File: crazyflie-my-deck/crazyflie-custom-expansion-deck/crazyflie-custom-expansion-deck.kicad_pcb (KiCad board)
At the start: 2 copper layers, 36.2 x 37.7 mm, 14 parts, among them J1 Conn_01x10, J2 Conn_01x06_Male, J3 Conn_01x10, U1 MAX712CSE

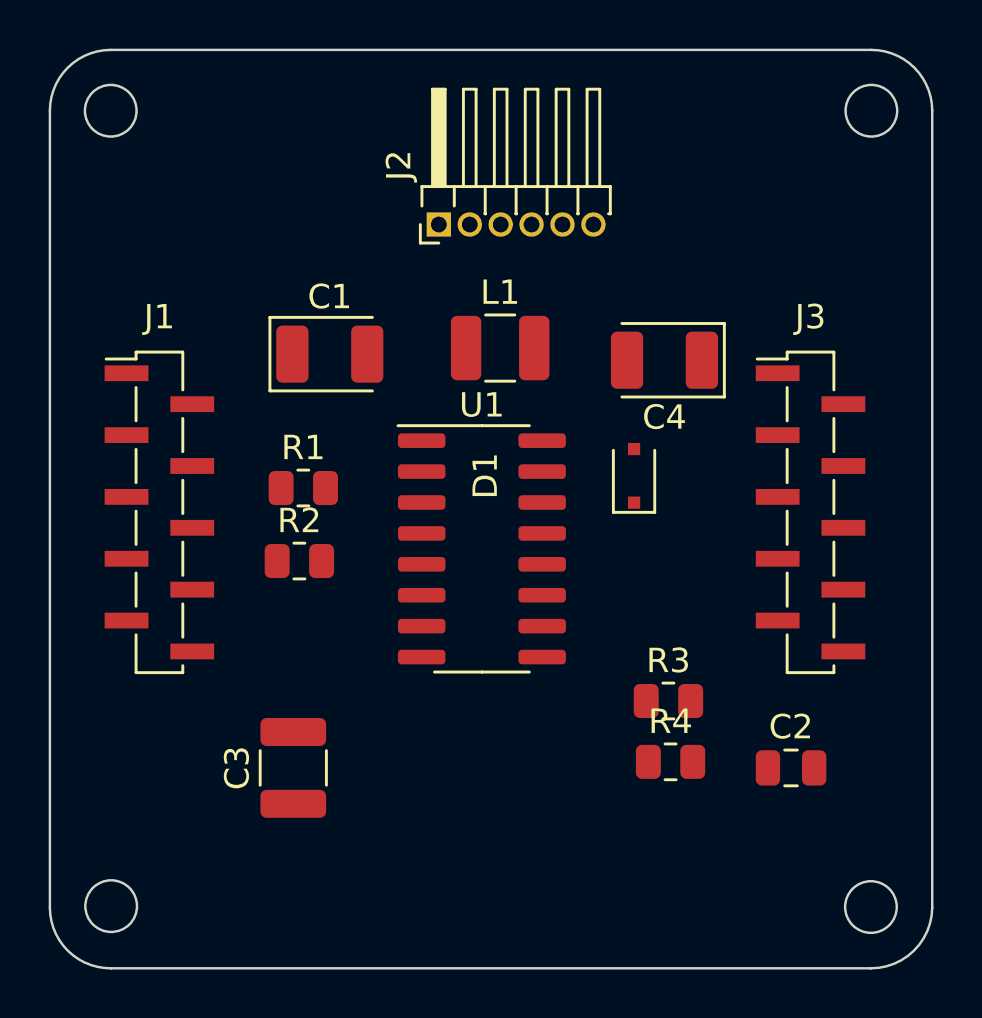
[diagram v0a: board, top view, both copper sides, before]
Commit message: Fixes
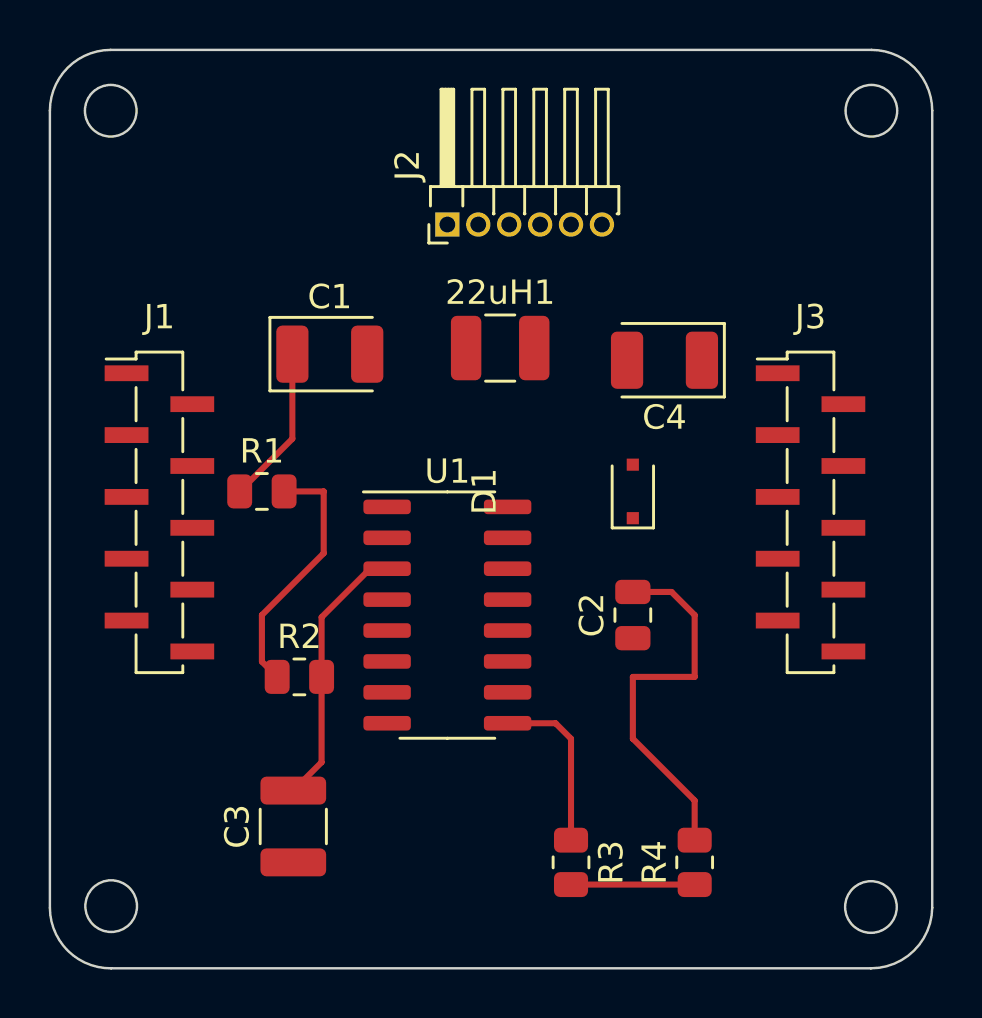
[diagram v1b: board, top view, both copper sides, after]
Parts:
- C1, C4: value C_Polarized -> 100uF
- C2: value C_Polarized -> 0.1uF
- C3: value C_Polarized -> 10uF
- R1: value R -> 120k
- R2: value R -> 30k
- R3: value R -> 390k
- R4: value R -> 130k
- U1: value MAX712CSE -> MAX7111
- moved C2 9.04 mm to (76.2, 45.7), turned to 90 degrees
- moved R3 7.74 mm to (73.7, 55.9), turned to -90 degrees
- moved R2 4.76 mm to (62.5, 48.3)
- moved R4 4.25 mm to (78.7, 55.9), turned to 90 degrees
- moved U1 3.07 mm to (68.6, 45.7)
- moved C3 2.41 mm to (62.2, 54.4)
- moved R1 1.71 mm to (61.0, 40.6)
- moved D1 0.64 mm to (76.2, 40.6)
- moved J2 0.35 mm to (68.6, 29.7)
- renumbered L1 to 22uH1
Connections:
- 22uH1 pad 2: Net-(D1-Pad2) -> Net-(22uH1-Pad2)
- C2 pad 1: unconnected-(C2-Pad1) -> Net-(C2-Pad1)
- C3 pad 1: unconnected-(C3-Pad1) -> Net-(C3-Pad1)
- D1 pad 2: Net-(D1-Pad2) -> Net-(22uH1-Pad2)
- R3 pad 1: unconnected-(R3-Pad1) -> Net-(C3-Pad1)
- U1 pad 1: unconnected-(U1-Pad1) -> Net-(22uH1-Pad2)
- U1 pad 10: unconnected-(U1-Pad10) -> Net-(C2-Pad1)
- U1 pad 11: unconnected-(U1-Pad11) -> Net-(R1-Pad2)
- U1 pad 12: unconnected-(U1-Pad12) -> Net-(C4-Pad1)
- U1 pad 13: unconnected-(U1-Pad13) -> Net-(C2-Pad1)
- U1 pad 14: unconnected-(U1-Pad14) -> GND
- U1 pad 15: unconnected-(U1-Pad15) -> GND
- U1 pad 16: unconnected-(U1-Pad16) -> Net-(22uH1-Pad2)
- U1 pad 2: unconnected-(U1-Pad2) -> GND
- U1 pad 3: unconnected-(U1-Pad3) -> GND
- U1 pad 4: unconnected-(U1-Pad4) -> Net-(C4-Pad1)
- U1 pad 5: unconnected-(U1-Pad5) -> Net-(C4-Pad1)
- U1 pad 6: unconnected-(U1-Pad6) -> Net-(R3-Pad2)
- U1 pad 7: unconnected-(U1-Pad7) -> Net-(C4-Pad1)
- U1 pad 9: unconnected-(U1-Pad9) -> Net-(C3-Pad1)
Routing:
- net GND: track 0.00 -> 26.9 mm
- net Net-(R1-Pad2): track 0.00 -> 10.6 mm
- net Net-(C3-Pad1): track 0.00 -> 7.04 mm
- net Net-(22uH1-Pad1): track 0.00 -> 6.54 mm
- net Net-(R3-Pad2): track 0.00 -> 5.08 mm
